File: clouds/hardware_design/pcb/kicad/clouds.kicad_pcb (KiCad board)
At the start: 2 copper layers, 88.9 x 106 mm, 150 parts, among them IC1 74595D, IC10 TL072D, IC2 LM1117-3.3, IC3 MCP6002, IC4 MCP6004, IC5 STM32F405RGT6, IC6 LM4040B10, IC7 LM1117-3.3, IC8 WM8731, IC9 TL072D, J1 PJ301_THONKICONN6, J10 PJ301_THONKICONN6, J11 PJ301_THONKICONN6, J12 PJ301_THONKICONN6, J2 PJ301_THONKICONN6, J3 PJ301_THONKICONN6, J4 PJ301_THONKICONN6, J5 PJ301_THONKICONN6, J6 PJ301_THONKICONN6, J7 PJ301_THONKICONN6, J8 PJ301_THONKICONN6, J9 PJ301_THONKICONN6, Q1 MMBT3904, Q2 MMBT3904, Q3 8MHz, Q4 12.288MHz, SW1 SW_Push_LED, SW2 TAC_SWITCHPTH, SW3 TAC_SWITCHPTH, SW4 EVQQ2, SW5 EVQQ2

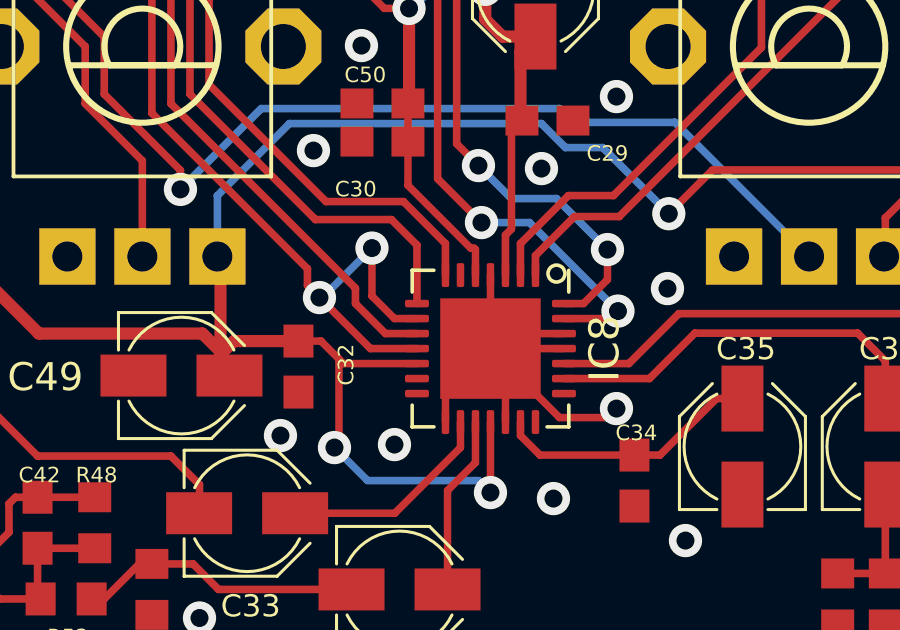
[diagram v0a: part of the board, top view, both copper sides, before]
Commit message: clouds cleanup
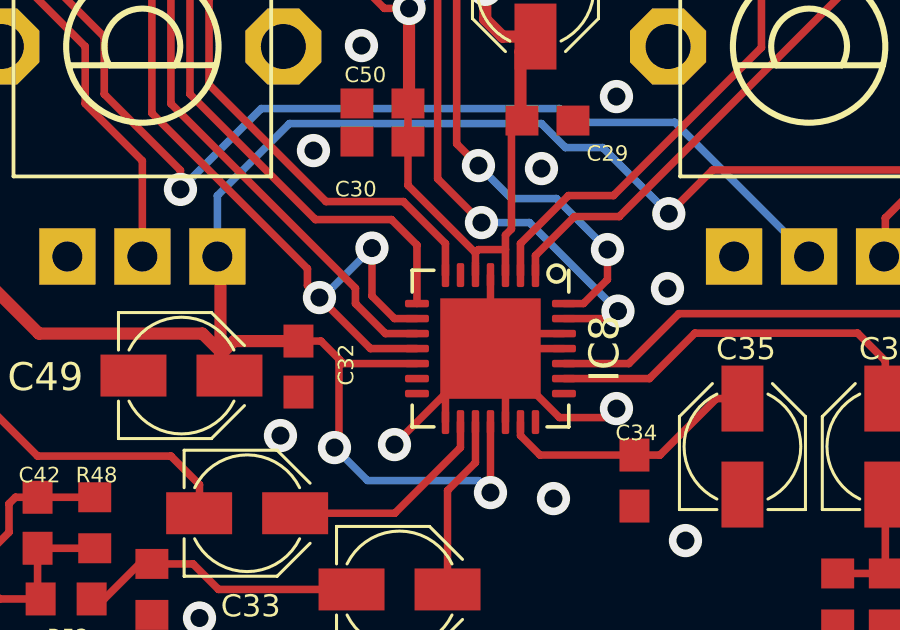
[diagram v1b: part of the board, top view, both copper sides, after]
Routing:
- net GND: track 15.0 -> 19.6 mm
- net +3V3: track 276.3 -> 277.3 mm
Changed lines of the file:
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@@
     (fp_arc (start 5.109 1.142899) (mid 4.379367 1.795994) (end 3.429 2.032) (layer "F.SilkS") (width 0.0508))
     (fp_arc (start -3.9826 -1.143) (mid -3.712991 -1.237845) (end -3.429 -1.27) (layer "F.SilkS") (width 0.0508))
-    (fp_arc (start 3.9826 1.143) (mid 3.712991 1.237849) (end 3.429 1.27) (layer "F.SilkS") (width 0.0508))
+    (fp_arc (start 3.9826 1.143) (mid 3.712989 1.237841) (end 3.429 1.27) (layer "F.SilkS") (width 0.0508))
     (fp_line (start -5.715 0.381) (end -5.715 -0.381) (layer "F.Fab") (width 0.1524))
     (fp_line (start 5.715 1.143) (end 5.715 -1.143) (layer "F.Fab") (width 0.1524))
@@
     (fp_arc (start -3.429 2.032001) (mid -4.379408 1.796063) (end -5.1091 1.143) (layer "F.SilkS") (width 0.0508))
     (fp_arc (start 5.461 -2.413) (mid 5.640605 -2.338605) (end 5.715 -2.159) (layer "F.SilkS") (width 0.1524))
-    (fp_arc (start 3.9826 1.143) (mid 3.712991 1.237849) (end 3.429 1.27) (layer "F.SilkS") (width 0.0508))
+    (fp_arc (start 3.9826 1.143) (mid 3.712989 1.237841) (end 3.429 1.27) (layer "F.SilkS") (width 0.0508))
     (fp_arc (start -3.429 1.27) (mid -3.712991 1.237845) (end -3.9826 1.143) (layer "F.SilkS") (width 0.0508))
     (fp_arc (start -5.715 -2.159) (mid -5.640605 -2.338605) (end -5.461 -2.413) (layer "F.SilkS") (width 0.1524))
@@
   (segment (start 170.9 119.2) (end 173.2 121.5) (width 0.25) (layer "F.Cu") (net 1))
   (segment (start 173.35 118.7) (end 171.4 118.7) (width 0.25) (layer "F.Cu") (net 1))
+  (segment (start 170.9 119.2) (end 167.7 122.4) (width 0.25) (layer "F.Cu") (net 1))
   (segment (start 169.4 121.65) (end 169.4 120.7) (width 0.25) (layer "F.Cu") (net 1))
   (segment (start 171.4 121.65) (end 171.4 119.7) (width 0.25) (layer "F.Cu") (net 1))
@@
   (segment (start 164.3761 85.0011) (end 163.1061 85.0011) (width 0.254) (layer "F.Cu") (net 96))
   (segment (start 162.43724 85.602144) (end 163.3821 86.5471) (width 0.254) (layer "F.Cu") (net 96))
-  (segment (start 170.245101 115.8568) (end 168.15 113.761699) (width 0.25) (layer "F.Cu") (net 96))
   (segment (start 171.6 111.95) (end 171.6 115.214527) (width 0.254) (layer "F.Cu") (net 96))
   (segment (start 154.5336 96.4311) (end 155.0895 96.4311) (width 0.254) (layer "F.Cu") (net 96))
+  (segment (start 170.4 116.011699) (end 168.15 113.761699) (width 0.25) (layer "F.Cu") (net 96))
   (segment (start 144.9061 74.8411) (end 143.4211 74.8411) (width 0.4064) (layer "F.Cu") (net 96))
   (segment (start 161.5186 100.6857) (end 160.84974 101.35456) (width 0.254) (layer "F.Cu") (net 96))
@@
   (segment (start 171.6 115.214527) (end 171.4 115.414527) (width 0.254) (layer "F.Cu") (net 96))
   (segment (start 147.7073 70.2374) (end 148.5011 69.4436) (width 0.3048) (layer "F.Cu") (net 96))
-  (segment (start 170.3568 115.8568) (end 170.245101 115.8568) (width 0.25) (layer "F.Cu") (net 96))
   (segment (start 165.3286 85.0011) (end 164.3761 85.0011) (width 0.4064) (layer "F.Cu") (net 96))
-  (segment (start 168.15 113.761699) (end 168.15 112.3) (width 0.25) (layer "F.Cu") (net 96))
   (segment (start 184.0611 76.4389) (end 184.0611 77.1661) (width 0.254) (layer "F.Cu") (net 96))
   (segment (start 173.5836 94.2086) (end 170.7305 94.2086) (width 0.254) (layer "F.Cu") (net 96))
@@
   (segment (start 147.1286 74.7386) (end 147.7073 74.1599) (width 0.4064) (layer "F.Cu") (net 96))
   (segment (start 170.7261 108.2261) (end 171.3 108.8) (width 0.4064) (layer "F.Cu") (net 96))
-  (segment (start 170.4 115.9) (end 170.3568 115.8568) (width 0.25) (layer "F.Cu") (net 96))
   (segment (start 140.8811 69.5836) (end 135.6611 69.5836) (width 0.4064) (layer "F.Cu") (net 96))
   (segment (start 173.5836 94.5261) (end 173.5836 94.2086) (width 0.254) (layer "F.Cu") (net 96))
   (segment (start 152.0961 96.0111) (end 153.5811 96.0111) (width 0.254) (layer "F.Cu") (net 96))
   (segment (start 171.3 108.8) (end 172.399996 108.8) (width 0.4064) (layer "F.Cu") (net 96))
+  (segment (start 170.4 116) (end 170.5 115.9) (width 0.25) (layer "F.Cu") (net 96))
   (segment (start 155.3273 69.4436) (end 155.9623 69.4436) (width 0.3048) (layer "F.Cu") (net 96))
   (segment (start 142.7861 70.3961) (end 141.9736 69.5836) (width 0.4064) (layer "F.Cu") (net 96))
   (segment (start 148.5011 69.4436) (end 152.7873 69.4436) (width 0.3048) (layer "F.Cu") (net 96))
-  (segment (start 171.4 115.414527) (end 171.4 116.75) (width 0.254) (layer "F.Cu") (net 96))
+  (segment (start 171.4 115.9) (end 171.4 116.75) (width 0.254) (layer "F.Cu") (net 96))
+  (segment (start 171.4 115.414527) (end 171.4 115.9) (width 0.254) (layer "F.Cu") (net 96))
   (segment (start 169.1386 76.1111) (end 169.1386 78.6511) (width 0.4064) (layer "F.Cu") (net 96))
   (segment (start 190.7 65.0247) (end 186.925 68.7997) (width 0.254) (layer "F.Cu") (net 96))
@@
   (segment (start 174.2186 64.3636) (end 180.8861 64.3636) (width 0.254) (layer "F.Cu") (net 96))
   (segment (start 163.3821 86.5471) (end 163.382115 86.724282) (width 0.254) (layer "F.Cu") (net 96))
-  (segment (start 170.4 116.75) (end 170.4 115.9) (width 0.25) (layer "F.Cu") (net 96))
   (segment (start 151.9936 96.1136) (end 152.0961 96.0111) (width 0.254) (layer "F.Cu") (net 96))
   (segment (start 161.5186 100.2411) (end 161.5186 100.6857) (width 0.254) (layer "F.Cu") (net 96))
@@
   (segment (start 166.7 107.2) (end 167.3611 107.8611) (width 0.25) (layer "F.Cu") (net 96))
   (segment (start 170.7305 94.2086) (end 170.061556 94.87756) (width 0.254) (layer "F.Cu") (net 96))
+  (segment (start 168.15 113.761699) (end 168.15 112.3) (width 0.25) (layer "F.Cu") (net 96))
   (segment (start 168.15 112.3) (end 168.15 111.03) (width 0.254) (layer "F.Cu") (net 96))
+  (segment (start 170.4 116.35) (end 170.4 116.011699) (width 0.25) (layer "F.Cu") (net 96))
   (segment (start 169.8 104.9) (end 170.7261 105.8261) (width 0.25) (layer "F.Cu") (net 96))
   (segment (start 168.1861 79.6036) (end 168.1861 82.1436) (width 0.4064) (layer "F.Cu") (net 96))
@@
   (segment (start 180.8861 64.3636) (end 180.8861 64.9986) (width 0.254) (layer "F.Cu") (net 96))
   (segment (start 141.9736 69.5836) (end 140.8811 69.5836) (width 0.4064) (layer "F.Cu") (net 96))
+  (segment (start 170.4 116.75) (end 170.4 116.35) (width 0.25) (layer "F.Cu") (net 96))
   (segment (start 186.925 68.7997) (end 186.925 73.6) (width 0.254) (layer "F.Cu") (net 96))
   (segment (start 169.1386 78.6511) (end 168.1861 79.6036) (width 0.4064) (layer "F.Cu") (net 96))
@@
   (segment (start 155.9623 69.4436) (end 156.9148 70.3961) (width 0.3048) (layer "F.Cu") (net 96))
   (segment (start 188.5061 94.2086) (end 189.1411 94.8436) (width 0.254) (layer "F.Cu") (net 96))
+  (segment (start 170.5 115.9) (end 171.4 115.9) (width 0.25) (layer "F.Cu") (net 96))
   (segment (start 181.2036 63.7286) (end 181.2036 61.8236) (width 0.254) (layer "F.Cu") (net 96))
   (segment (start 172.399996 108.8) (end 171.9 109.299996) (width 0.4064) (layer "F.Cu") (net 96))
